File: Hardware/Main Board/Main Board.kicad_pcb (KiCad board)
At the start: 2 copper layers, 54 parts, among them Q1 MMBT3904-TP, Q2 MMBT3904-TP, Q3 AO4484, SW1 Momentary, U1 MT3608, U2 NCP718A, U3 ATtiny1614, U4 TP4056

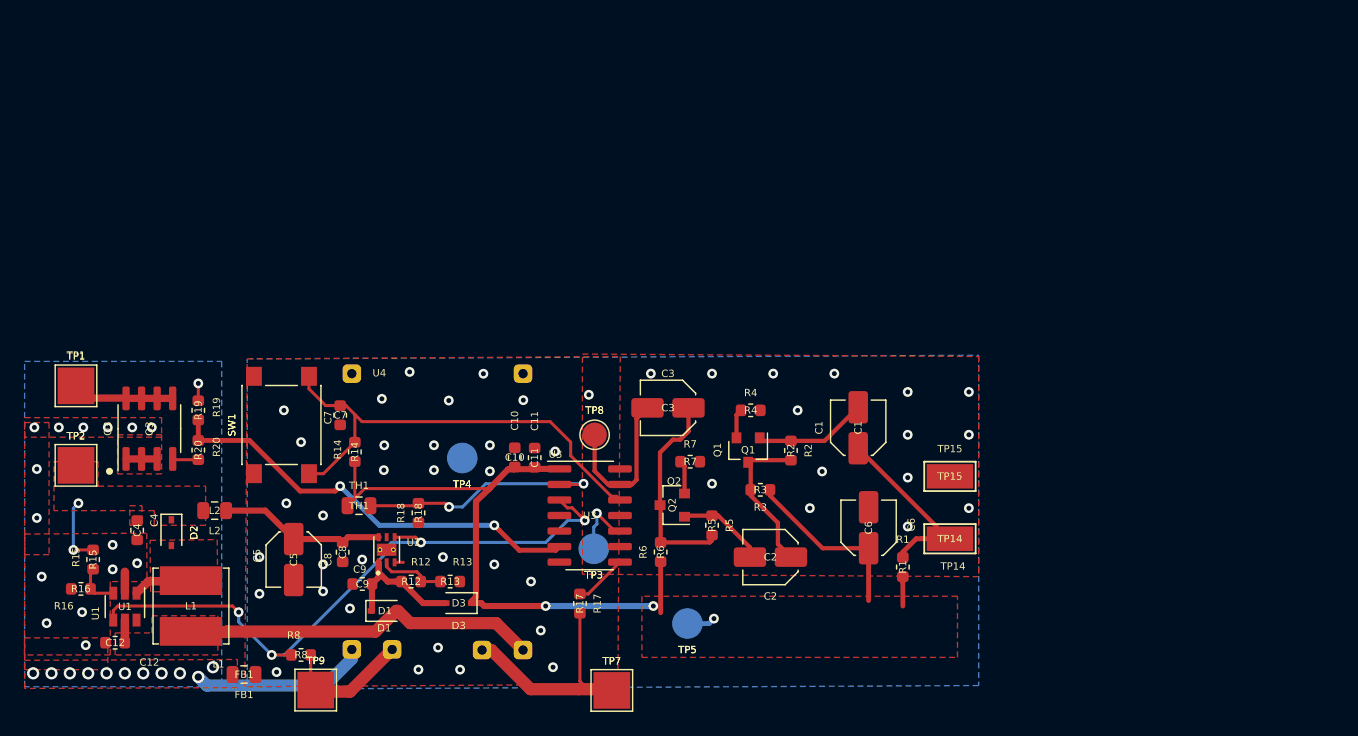
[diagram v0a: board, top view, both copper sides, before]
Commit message: PCB completed and ready for reviewgit add .git add .
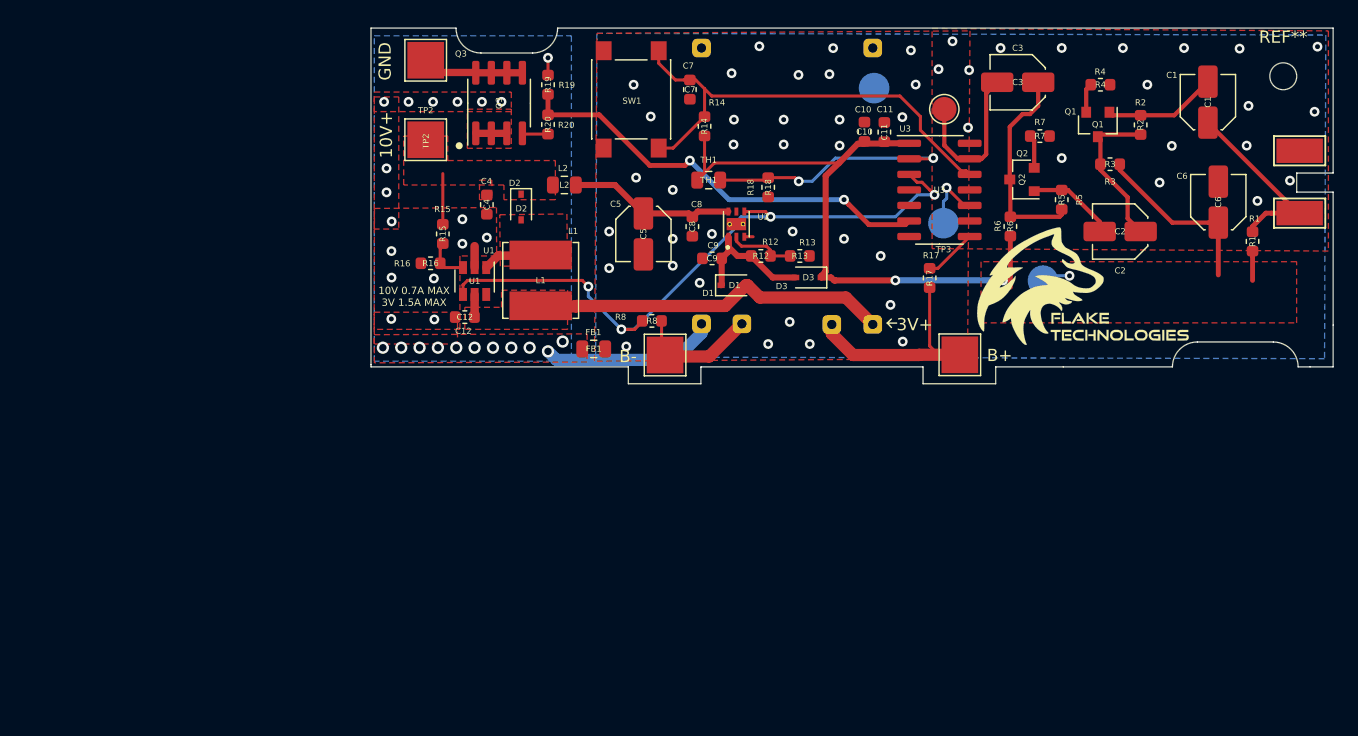
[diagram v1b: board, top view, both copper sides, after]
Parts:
- added G***: LOGO, 1, F.Cu at (165.8, 105.3)
- added G***: LOGO, 123332343423, B.Cu at (139.7, 93.5)
- added G***: LOGO, 3333, B.Cu at (180.5, 101.7)
- added G***: LOGO, ddr, F.Cu at (0.00, 0.00)
- added REF**: MountingHole_2.2mm_M2, MountingHole:MountingHole_2.2mm_M2, F.Cu at (181.7, 87.7)
- moved TP4 45.3 mm to (148.2, 88.7)
- moved TP5 40.4 mm to (162.1, 104.4)
- moved R8 39.6 mm to (130.1, 107.7)
- moved TP9 39.6 mm to (131.2, 110.5)
- moved TP7 39.5 mm to (155.3, 110.5)
- moved C11 39.1 mm to (149.1, 92.3)
- moved C12 39.1 mm to (114.8, 107.4)
- moved C2 39.1 mm to (168.4, 100.4)
- moved C7 39.1 mm to (133.2, 88.8)
- moved D2 39.1 mm to (119.4, 98.4)
- moved Q1 39.1 mm to (166.5, 91.6)
- moved Q2 39.1 mm to (160.3, 96.1)
- moved Q3 39.1 mm to (117.6, 89.9)
- moved R1 39.1 mm to (179.2, 101.2)
- moved R12 39.1 mm to (139.0, 102.4)
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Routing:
- net +10V: track 5.86 -> 4.14 mm, vias 2 -> 0
- net GNDREF: track 10.8 -> 10.3 mm
- net GNDPWR: vias 27 -> 29
- net GNDA: vias 47 -> 52
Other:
- board outline added: 78.7 x 29.1 mm
- board text added: "10V 0.7A MAX 3V 1.5A MAX"
- board text added: "10V+"
- board text added: "3V+"
- board text added: "B+"
- board text added: "B-"
- board text added: "DAVID "DDR" ROBERTS"
- board text added: "G"
- board text added: "GND"
- board text added: "MICHAEL "CORNFLAKES" MADI"
- board text added: "PGM"
- board text added: "V"
